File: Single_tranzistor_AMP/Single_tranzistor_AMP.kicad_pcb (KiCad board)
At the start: 2 copper layers, 11 parts, among them J1 AC Input, J2 AC Output, Q1 2N4401

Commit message: Treniņuzdevums
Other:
- copper layers 2 -> 4
- net class Power added: clearance 0.2, trace_width 0.75, via_dia 0.8, via_drill 0.4
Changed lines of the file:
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@@
   )
   (page A4)
+  (title_block
+    (title Single_Transistor_AMP)
+    (date 2020-12-09)
+    (rev V1.0)
+    (company VeA)
+    (comment 1 A.Smirnova)
+  )
   (layers
     (0 F.Cu signal)
+    (1 In1.Cu power)
+    (2 In2.Cu power)
     (31 B.Cu signal)
     (32 B.Adhes user)
@@
     (solder_mask_min_width 0.25)
     (aux_axis_origin 0 0)
-    (visible_elements FFFFFF7F)
+    (visible_elements 7FFFFFFF)
     (pcbplotparams
       (layerselection 0x010fc_ffffffff)
@@
     (add_net "Net-(Q1-Pad3)")
   )
+  (net_class Power ""
+    (clearance 0.2)
+    (trace_width 0.75)
+    (via_dia 0.8)
+    (via_drill 0.4)
+    (uvia_dia 0.3)
+    (uvia_drill 0.1)
+  )
   (module Capacitor_THT:CP_Axial_L11.0mm_D5.0mm_P18.00mm_Horizontal (layer F.Cu)

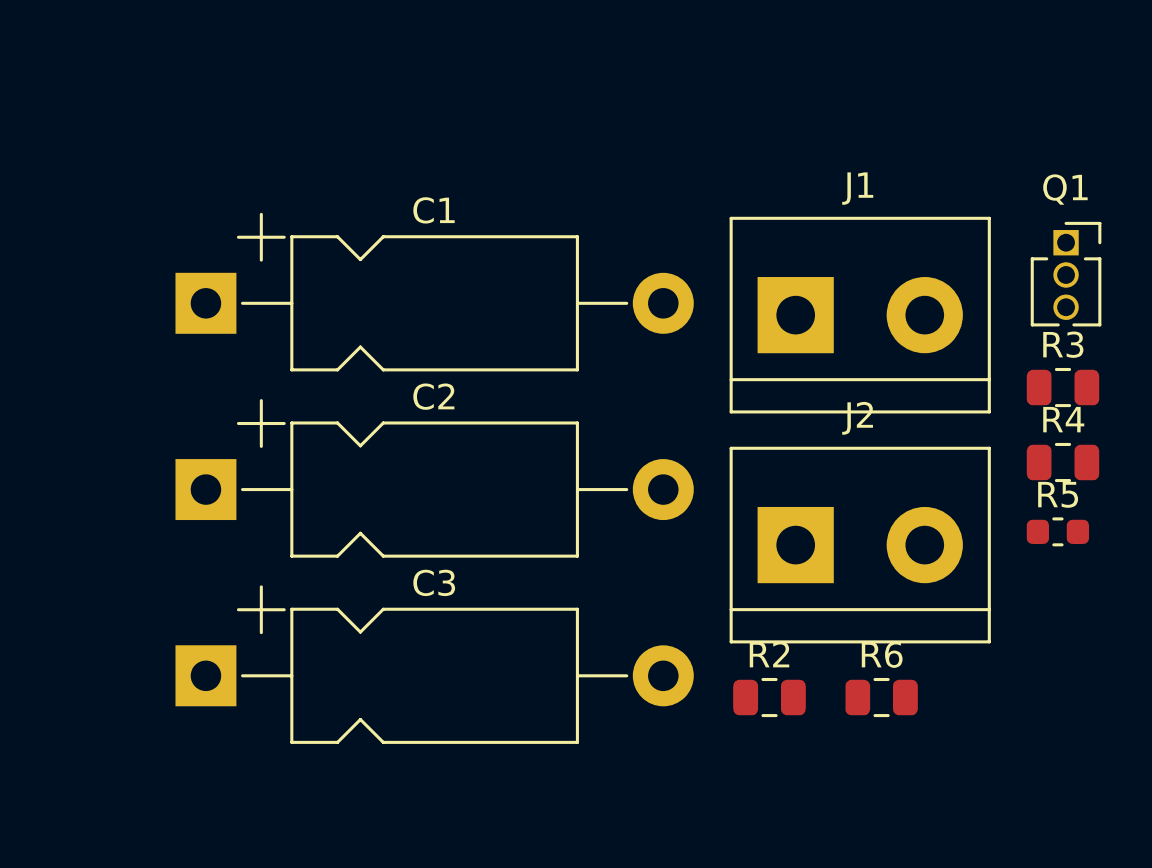
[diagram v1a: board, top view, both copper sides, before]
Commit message: LayOut
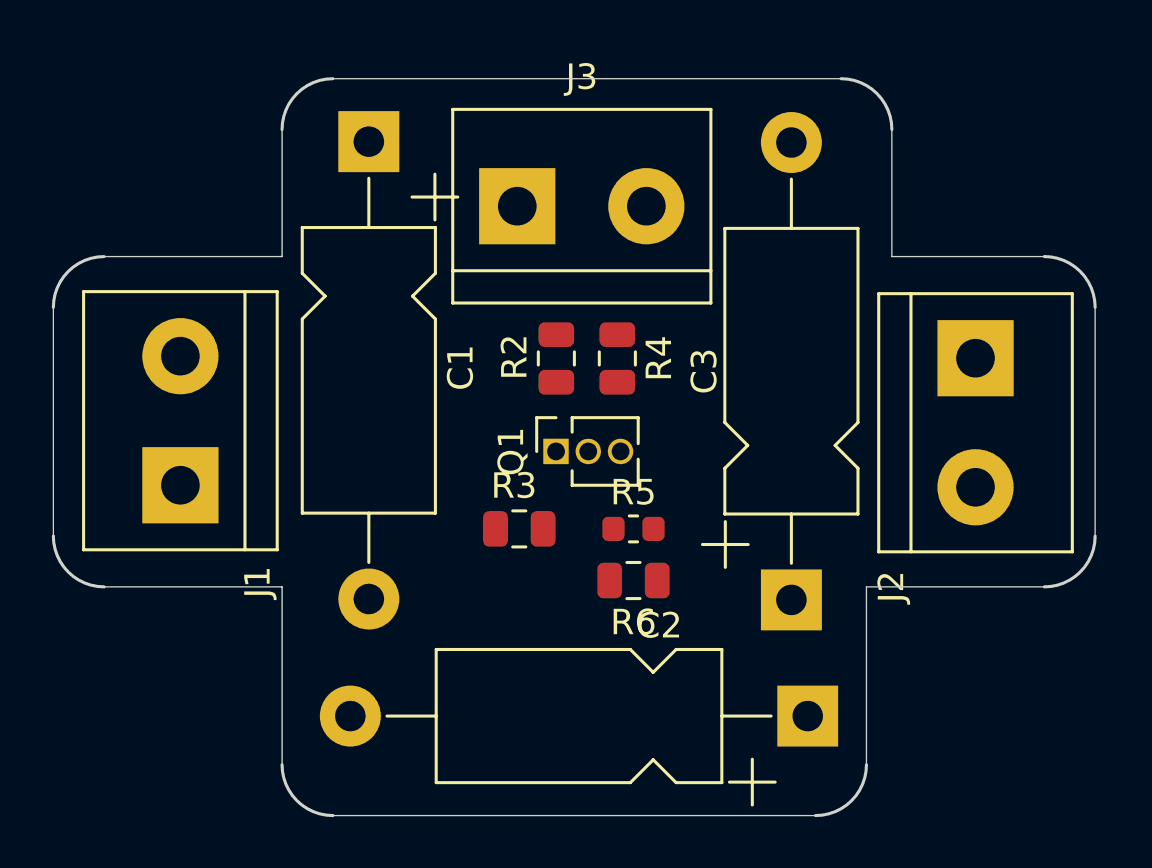
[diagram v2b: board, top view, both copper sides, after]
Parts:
- added J3: Power, TerminalBlock:TerminalBlock_bornier-2_P5.08mm, F.Cu at (33.3, 18.0)
- moved C2 25.3 mm to (44.7, 38.1), turned to 180 degrees
- moved J1 25.1 mm to (20.0, 29.0), turned to 90 degrees
- moved C3 23.2 mm to (44.0, 33.5), turned to 90 degrees
- moved R3 22.1 mm to (33.3, 30.7), turned to 180 degrees
- moved Q1 21.7 mm to (34.8, 27.7), turned to 90 degrees
- moved R4 18.0 mm to (37.2, 24.0), turned to 270 degrees
- moved R5 16.7 mm to (37.8, 30.7)
- moved R2 15.8 mm to (34.8, 24.0), turned to 270 degrees
- moved R6 10.8 mm to (37.8, 32.8), turned to 180 degrees
- moved J2 10.2 mm to (51.3, 24.0), turned to 270 degrees
- moved C1 9.03 mm to (27.4, 15.5), turned to 270 degrees
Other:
- board outline added: 41 x 29 mm
- copper layers 4 -> 2

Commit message: trasēšana
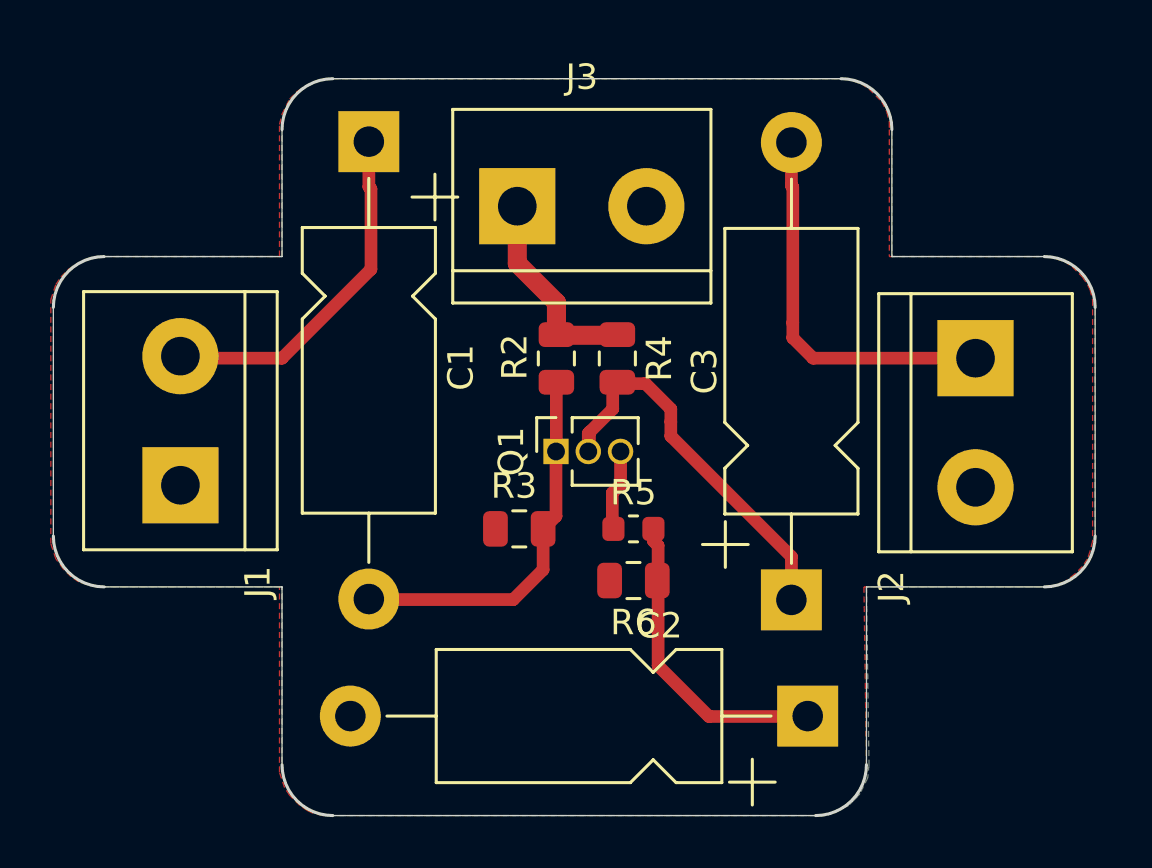
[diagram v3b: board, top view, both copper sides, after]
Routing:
- net Net-(C3-Pad1): track 0.00 -> 15.6 mm
- net Net-(C1-Pad2): track 0.00 -> 15.3 mm
- net Net-(C3-Pad2): track 0.00 -> 15.0 mm
- net Net-(C1-Pad1): track 0.00 -> 14.0 mm
- net Net-(C2-Pad1): track 0.00 -> 12.2 mm
- net +12V: track 0.00 -> 8.22 mm
- net Net-(Q1-Pad3): track 0.00 -> 3.26 mm
- added copper zone on B.Cu, net GND
- added copper zone on F.Cu, net GND
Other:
- net class Default: trace_width 0.25 -> 0.5
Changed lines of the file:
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@@
     (thickness 2)
     (drawings 20)
-    (tracks 0)
+    (tracks 42)
     (zones 0)
     (modules 12)
@@
   )
   (setup
-    (last_trace_width 0.25)
+    (last_trace_width 0.5)
     (user_trace_width 0.5)
     (user_trace_width 0.75)
@@
   (net_class Default "This is the default net class."
     (clearance 0.2)
-    (trace_width 0.25)
+    (trace_width 0.5)
     (via_dia 0.8)
     (via_drill 0.4)
     (uvia_dia 0.3)
     (uvia_drill 0.1)
-    (add_net +12V)
-    (add_net GND)
     (add_net "Net-(C1-Pad1)")
     (add_net "Net-(C1-Pad2)")
@@
     (uvia_dia 0.3)
     (uvia_drill 0.1)
+    (add_net +12V)
+    (add_net GND)
   )
   (module Capacitor_THT:CP_Axial_L11.0mm_D5.0mm_P18.00mm_Horizontal (layer F.Cu)
@@
   (gr_arc (start 54 31) (end 54 33) (angle -90) (layer Edge.Cuts) (width 0.12))
   (gr_arc (start 54 22) (end 56 22) (angle -90) (layer Edge.Cuts) (width 0.12))
+  (segment (start 27.416 17.255765) (end 27.5 17.339765) (width 0.5) (layer F.Cu) (net 1))
+  (segment (start 27.416 15.478) (end 27.416 17.255765) (width 0.5) (layer F.Cu) (net 1))
+  (segment (start 27.5 17.339765) (end 27.5 20.5) (width 0.5) (layer F.Cu) (net 1))
+  (segment (start 27.5 20.5) (end 24 24) (width 0.5) (layer F.Cu) (net 1))
+  (segment (start 24 24) (end 20 24) (width 0.5) (layer F.Cu) (net 1))
+  (segment (start 34.796 24.9475) (end 34.796 27.696) (width 0.5) (layer F.Cu) (net 2))
+  (segment (start 34.796 27.696) (end 34.8 27.7) (width 0.5) (layer F.Cu) (net 2))
+  (segment (start 34.782 27.67) (end 34.782 30.218) (width 0.5) (layer F.Cu) (net 2))
+  (segment (start 34.782 30.218) (end 34.3 30.7) (width 0.5) (layer F.Cu) (net 2))
+  (segment (start 34.274 30.718) (end 34.274 32.326) (width 0.5) (layer F.Cu) (net 2))
+  (segment (start 34.274 32.326) (end 33.1 33.5) (width 0.5) (layer F.Cu) (net 2))
+  (segment (start 33.1 33.5) (end 27.2 33.5) (width 0.5) (layer F.Cu) (net 2))
+  (segment (start 27.2 33.5) (end 27.3 33.5) (width 0.5) (layer F.Cu) (net 2))
+  (segment (start 38.6175 31.193) (end 38.8 31.3755) (width 0.5) (layer F.Cu) (net 4))
+  (segment (start 38.6175 30.718) (end 38.6175 31.193) (width 0.5) (layer F.Cu) (net 4))
+  (segment (start 38.8 31.3755) (end 38.8 32.9) (width 0.5) (layer F.Cu) (net 4))
+  (segment (start 38.8 32.9) (end 38.8 36.1) (width 0.5) (layer F.Cu) (net 4))
+  (segment (start 38.8 36.1) (end 40.8 38.1) (width 0.5) (layer F.Cu) (net 4))
+  (segment (start 40.8 38.1) (end 44.7 38.1) (width 0.5) (layer F.Cu) (net 4))
+  (segment (start 44.046 31.812) (end 39.3 27.066) (width 0.5) (layer F.Cu) (net 5))
+  (segment (start 44.046 33.512) (end 44.046 31.812) (width 0.5) (layer F.Cu) (net 5))
+  (segment (start 39.3 26) (end 38.3 25) (width 0.5) (layer F.Cu) (net 5))
+  (segment (start 38.3 25) (end 37.3 25) (width 0.5) (layer F.Cu) (net 5))
+  (segment (start 36.1 26.9) (end 36.1 27.6) (width 0.5) (layer F.Cu) (net 5))
+  (segment (start 39.3 26.5) (end 39.3 26) (width 0.5) (layer F.Cu) (net 5))
+  (segment (start 39.3 27.066) (end 39.3 26.5) (width 0.5) (layer F.Cu) (net 5))
+  (segment (start 36.052 26.962894) (end 37.014894 26) (width 0.5) (layer F.Cu) (net 5))
+  (segment (start 36.052 27.67) (end 36.052 26.962894) (width 0.5) (layer F.Cu) (net 5))
+  (segment (start 37.014894 26) (end 37.014894 25.014894) (width 0.5) (layer F.Cu) (net 5))
+  (segment (start 44.046 17.209056) (end 44.1 17.263056) (width 0.5) (layer F.Cu) (net 6))
+  (segment (start 44.046 15.512) (end 44.046 17.209056) (width 0.5) (layer F.Cu) (net 6))
+  (segment (start 44.1 17.263056) (end 44.1 22.6) (width 0.5) (layer F.Cu) (net 6))
+  (segment (start 44.1 22.6) (end 44.1 23.2) (width 0.5) (layer F.Cu) (net 6))
+  (segment (start 44.1 23.2) (end 44.9 24) (width 0.5) (layer F.Cu) (net 6))
+  (segment (start 44.9 24) (end 51.1 24) (width 0.5) (layer F.Cu) (net 6))
+  (segment (start 37.322 27.67) (end 37.322 28.978) (width 0.5) (layer F.Cu) (net 7))
+  (segment (start 37.322 28.978) (end 37 29.3) (width 0.5) (layer F.Cu) (net 7))
+  (segment (start 37 29.3) (end 37 30.8) (width 0.5) (layer F.Cu) (net 7))
+  (segment (start 33.258 20.268) (end 34.8 21.81) (width 0.75) (layer F.Cu) (net 8))
+  (segment (start 33.258 18.018) (end 33.258 20.268) (width 0.75) (layer F.Cu) (net 8))
+  (segment (start 34.8 21.81) (end 34.8 23.1) (width 0.75) (layer F.Cu) (net 8))
+  (segment (start 34.8 23.1) (end 37.3 23.1) (width 0.75) (layer F.Cu) (net 8))
+  (zone (net 3) (net_name GND) (layer F.Cu) (hatch edge 0.508)
+    (connect_pads (clearance 0.508))
+    (min_thickness 0.254)
+    (fill yes (arc_segments 32) (thermal_gap 0.508) (thermal_bridge_width 0.508))
+    (polygon
+      (pts
+        (xy 46.5 13.1) (xy 46.8 13.2) (xy 47.1 13.4) (xy 47.6 13.9) (xy 47.8 14.3)
+        (xy 47.9 14.7) (xy 47.9 15) (xy 47.9 20) (xy 54.1 20) (xy 54.5 20.1)
+        (xy 54.8 20.2) (xy 55.1 20.4) (xy 55.5 20.8) (xy 55.7 21.1) (xy 55.8 21.3)
+        (xy 55.9 21.7) (xy 55.9 31.2) (xy 55.8 31.6) (xy 55.7 31.9) (xy 55.5 32.2)
+        (xy 55.2 32.5) (xy 54.8 32.8) (xy 54.2 33) (xy 46.9 33) (xy 47 40)
+        (xy 46.95 40.5125) (xy 46.65 41.125) (xy 46.5 41.3) (xy 46.4 41.4) (xy 46.2 41.6)
+        (xy 45.6 41.9) (xy 45.3 42) (xy 25.6 42) (xy 25.2 41.9) (xy 25 41.8)
+        (xy 24.7 41.6) (xy 24.3 41.2) (xy 24.1 40.9) (xy 23.9 40.3) (xy 23.9 33)
+        (xy 16.7 33) (xy 16.3 32.9) (xy 16 32.8) (xy 15.7 32.6) (xy 15.4 32.3)
+        (xy 15.1 31.9) (xy 14.9 31.3) (xy 14.9 21.7) (xy 15.1 21.1) (xy 15.3 20.8)
+        (xy 15.6 20.5) (xy 15.9 20.3) (xy 16.3 20.1) (xy 16.6 20) (xy 23.9 20)
+        (xy 23.9 14.8) (xy 24 14.4) (xy 24.3 13.8) (xy 24.6 13.5) (xy 24.9 13.3)
+        (xy 25.3 13.1) (xy 25.6 13) (xy 46.1 13)
+      )
+    )
+  )
+  (zone (net 3) (net_name GND) (layer B.Cu) (hatch edge 0.508)
+    (connect_pads (clearance 0.508))
+    (min_thickness 0.254)
+    (fill yes (arc_segments 32) (thermal_gap 0.508) (thermal_bridge_width 0.508))
+    (polygon
+      (pts
+        (xy 46.6 13.1) (xy 46.9 13.2) (xy 47.2 13.4) (xy 47.7 13.9) (xy 47.9 14.3)
+        (xy 48 14.7) (xy 48 15) (xy 48 20) (xy 54.2 20) (xy 54.6 20.1)
+        (xy 54.9 20.2) (xy 55.2 20.4) (xy 55.6 20.8) (xy 55.8 21.1) (xy 55.9 21.3)
+        (xy 56 21.7) (xy 56 31.2) (xy 55.9 31.6) (xy 55.8 31.9) (xy 55.6 32.2)
+        (xy 55.3 32.5) (xy 54.9 32.8) (xy 54.3 33) (xy 47 33) (xy 47.1 40)
+        (xy 47.05 40.5125) (xy 46.75 41.125) (xy 46.6 41.3) (xy 46.5 41.4) (xy 46.3 41.6)
+        (xy 45.7 41.9) (xy 45.4 42) (xy 25.7 42) (xy 25.3 41.9) (xy 25.1 41.8)
+        (xy 24.8 41.6) (xy 24.4 41.2) (xy 24.2 40.9) (xy 24 40.3) (xy 24 33)
+        (xy 16.8 33) (xy 16.4 32.9) (xy 16.1 32.8) (xy 15.8 32.6) (xy 15.5 32.3)
+        (xy 15.2 31.9) (xy 15 31.3) (xy 15 21.7) (xy 15.2 21.1) (xy 15.4 20.8)
+        (xy 15.7 20.5) (xy 16 20.3) (xy 16.4 20.1) (xy 16.7 20) (xy 24 20)
+        (xy 24 14.8) (xy 24.1 14.4) (xy 24.4 13.8) (xy 24.7 13.5) (xy 25 13.3)
+        (xy 25.4 13.1) (xy 25.7 13) (xy 46.2 13)
+      )
+    )
+  )
 )
